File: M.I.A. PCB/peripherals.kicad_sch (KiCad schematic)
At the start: 22 parts, among them J10 Conn_01x03, J11 Conn_01x03, J12 Conn_Coaxial, J3 Conn_01x03, J4 Conn_01x03, J5 Conn_01x03, J6 Conn_01x03, J7 MSD-4-A, J8 Conn_01x03, J9 Conn_01x03, U15 74AHC541, U16 RFM95W-915S2

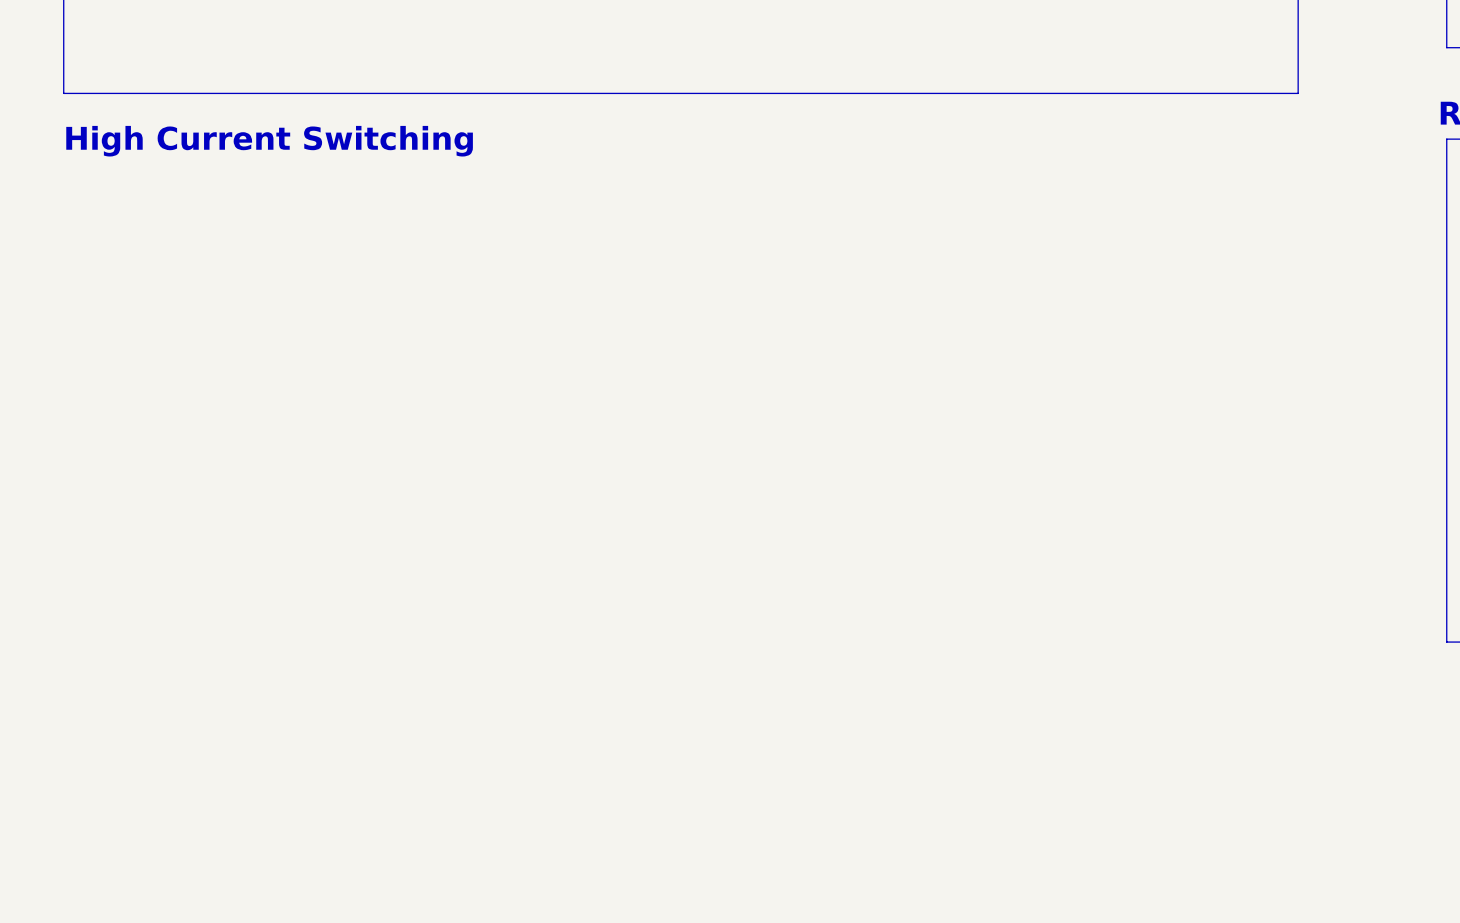
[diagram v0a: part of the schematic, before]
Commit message: Worked on Layout, Changed IMU
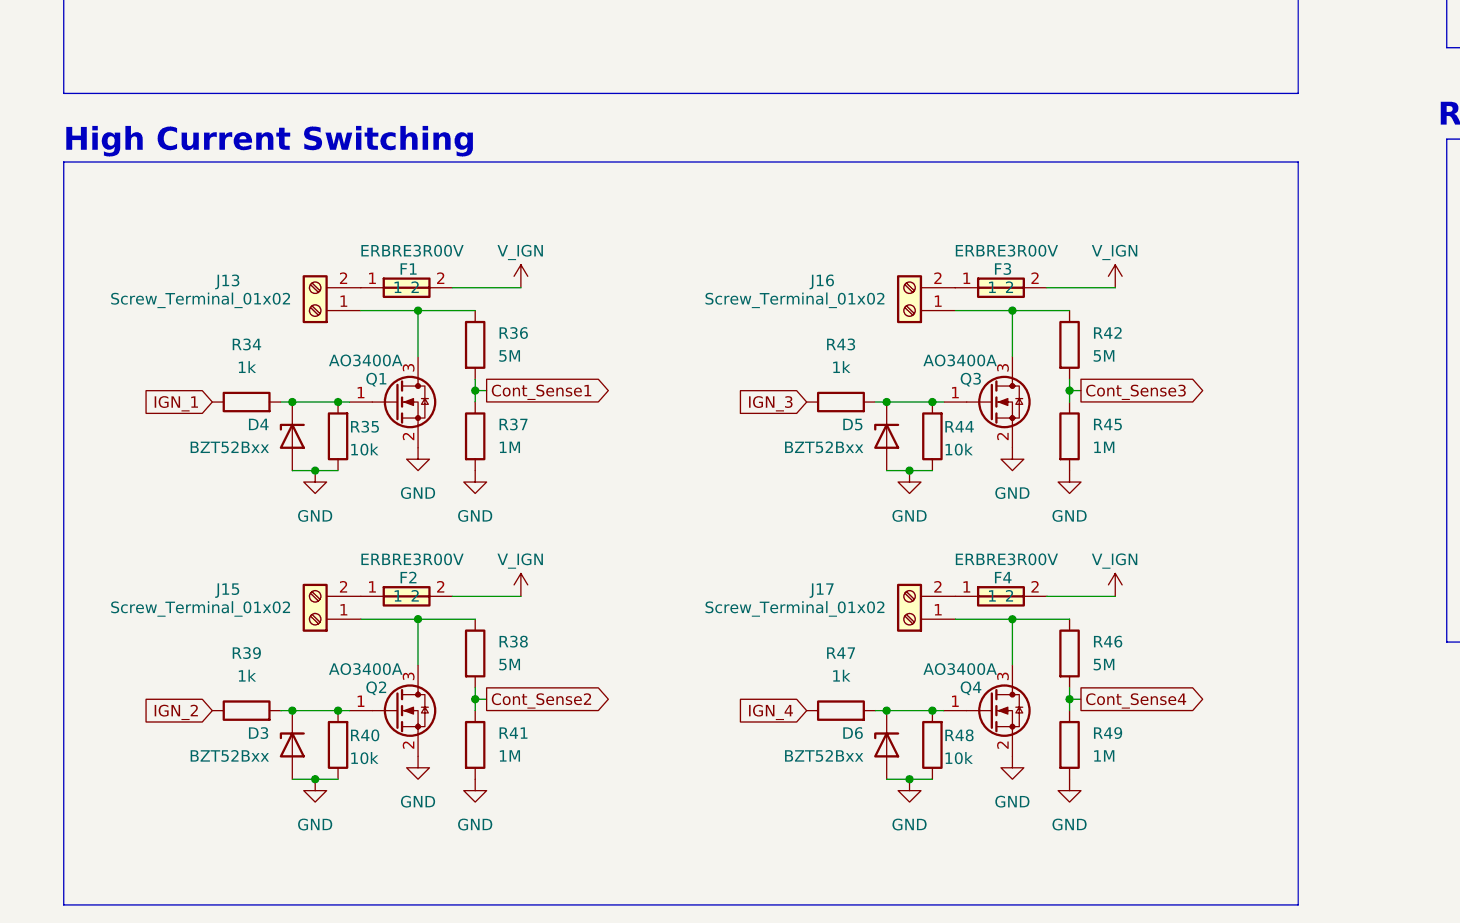
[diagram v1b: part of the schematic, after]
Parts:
- added D3, D4, D5, D6: BZT52Bxx, Diode_SMD:D_SOD-123F, symbol Diode:BZT52Bxx
- added F1, F2, F3, F4: ERBRE3R00V, JLCImport:ERBRE3R00V, symbol JLCImport:ERBRE3R00V
- added J13, J15, J16, J17: Screw_Terminal_01x02, TerminalBlock_Phoenix:TerminalBlock_Phoenix_MKDS-1-2-3.81_1x02_P3.81mm_Horizontal, symbol Connector:Screw_Terminal_01x02
- added Q1, Q2, Q3, Q4: AO3400A, Package_TO_SOT_SMD:SOT-23, symbol Transistor_FET:AO3400A
- added R34, R39, R43, R47: 1k, Resistor_SMD:R_0603_1608Metric, symbol Device:R
- added R35, R40, R44, R48: 10k, Resistor_SMD:R_0603_1608Metric, symbol Device:R
- added R36, R38, R42, R46: 5M, Resistor_SMD:R_0603_1608Metric, symbol Device:R
- added R37, R41, R45, R49: 1M, Resistor_SMD:R_0603_1608Metric, symbol Device:R
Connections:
- net GND: now also D3.2 (A), D4.2 (A), D5.2 (A), D6.2 (A), Q1.2 (S), Q2.2 (S), Q3.2 (S), Q4.2 (S), R35.1, R37.2, R40.1, R41.2, R44.1, R45.2, R48.1, R49.2
- new net: D5.1 (K), Q3.1 (G), R43.2, R44.2
- new net: F1.1, J13.2 (Pin_2)
- new net: D4.1 (K), Q1.1 (G), R34.2, R35.2
- new net: D3.1 (K), Q2.1 (G), R39.2, R40.2
- new net: D6.1 (K), Q4.1 (G), R47.2, R48.2
- new net: J15.1 (Pin_1), Q2.3 (D), R38.1
- new net: J16.1 (Pin_1), Q3.3 (D), R42.1
- new net: J17.1 (Pin_1), Q4.3 (D), R46.1
- new net: F4.1, J17.2 (Pin_2)
- new net: F3.1, J16.2 (Pin_2)
- new net: F2.1, J15.2 (Pin_2)
- new net: J13.1 (Pin_1), Q1.3 (D), R36.1
- new net Cont_Sense1: R36.2, R37.1
- new net Cont_Sense2: R38.2, R41.1
- new net Cont_Sense3: R42.2, R45.1
- new net Cont_Sense4: R46.2, R49.1
- new net IGN_1: R34.1
- new net IGN_2: R39.1
- new net IGN_3: R43.1
- new net IGN_4: R47.1
- new net V_IGN: F1.2, F2.2, F3.2, F4.2
